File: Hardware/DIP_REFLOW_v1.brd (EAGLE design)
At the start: 78.7 x 78.4 mm, 32 parts, among them IC1 7805, J1 ICSP, Q1 2N3904, Q2 2N3904, Q3 2N3904, U1 ATMEGA328P_PDIP, U2 LCD-16X2SILK, Y1 16Mhz

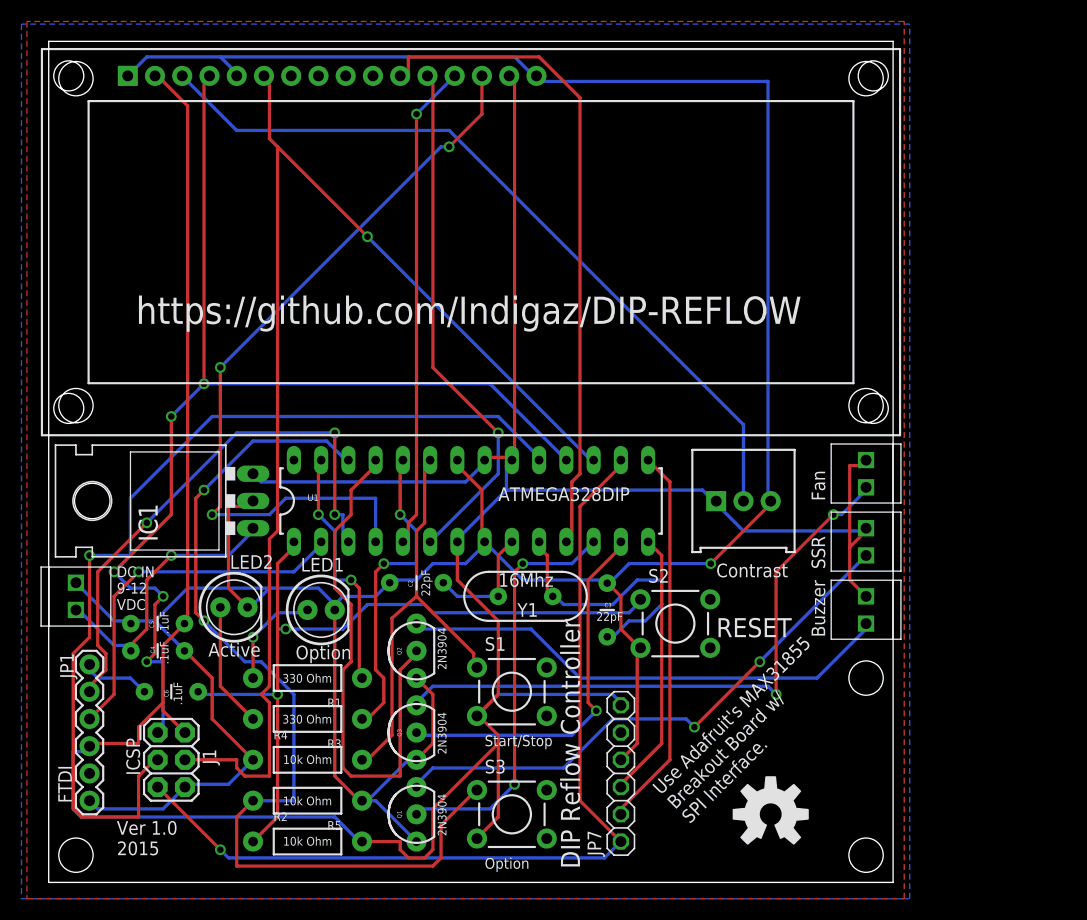
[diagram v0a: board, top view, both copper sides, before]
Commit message: Updates and Fixes
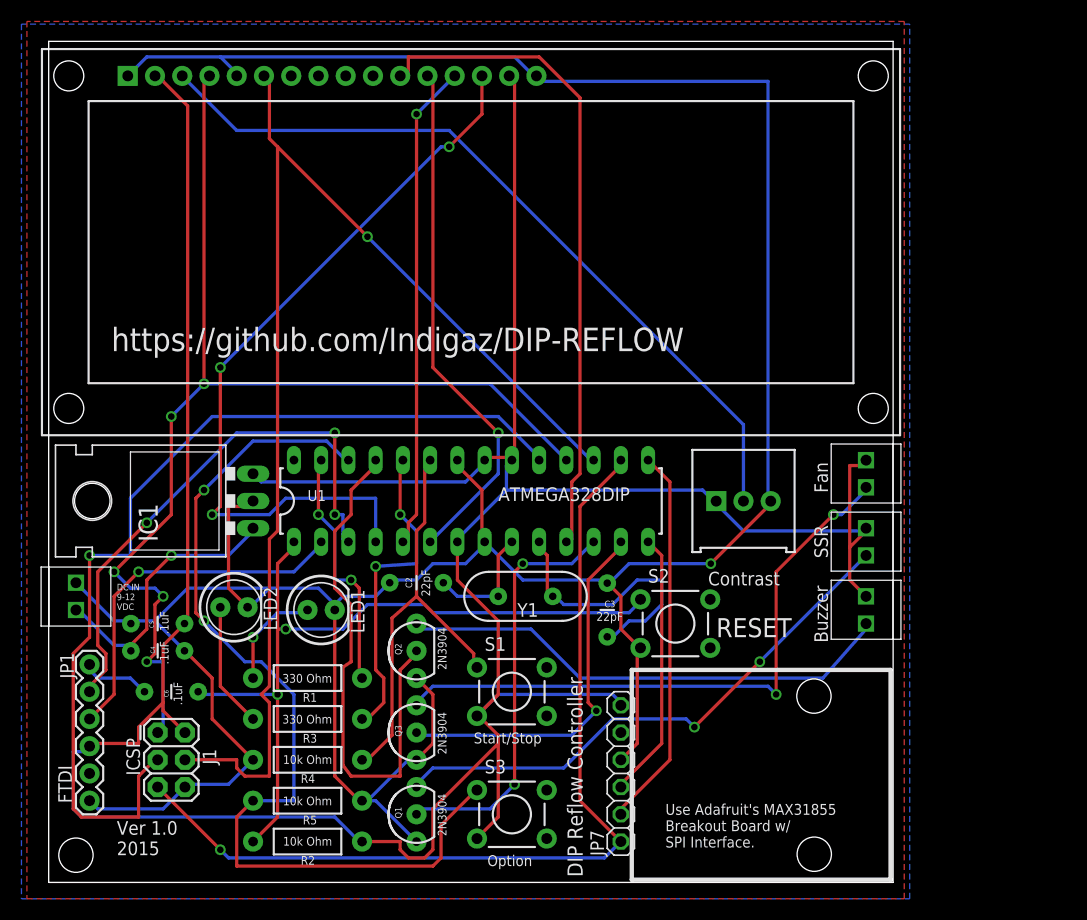
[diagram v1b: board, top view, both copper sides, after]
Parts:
- removed LOGO1: OSHW-LOGOL, SparkFun-Aesthetics:OSHW-LOGO-L
